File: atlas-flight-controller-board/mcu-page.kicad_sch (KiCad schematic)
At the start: 5 parts, among them J1 LED Indicator Header, J4 5V Input Power, U2 DEV-16771

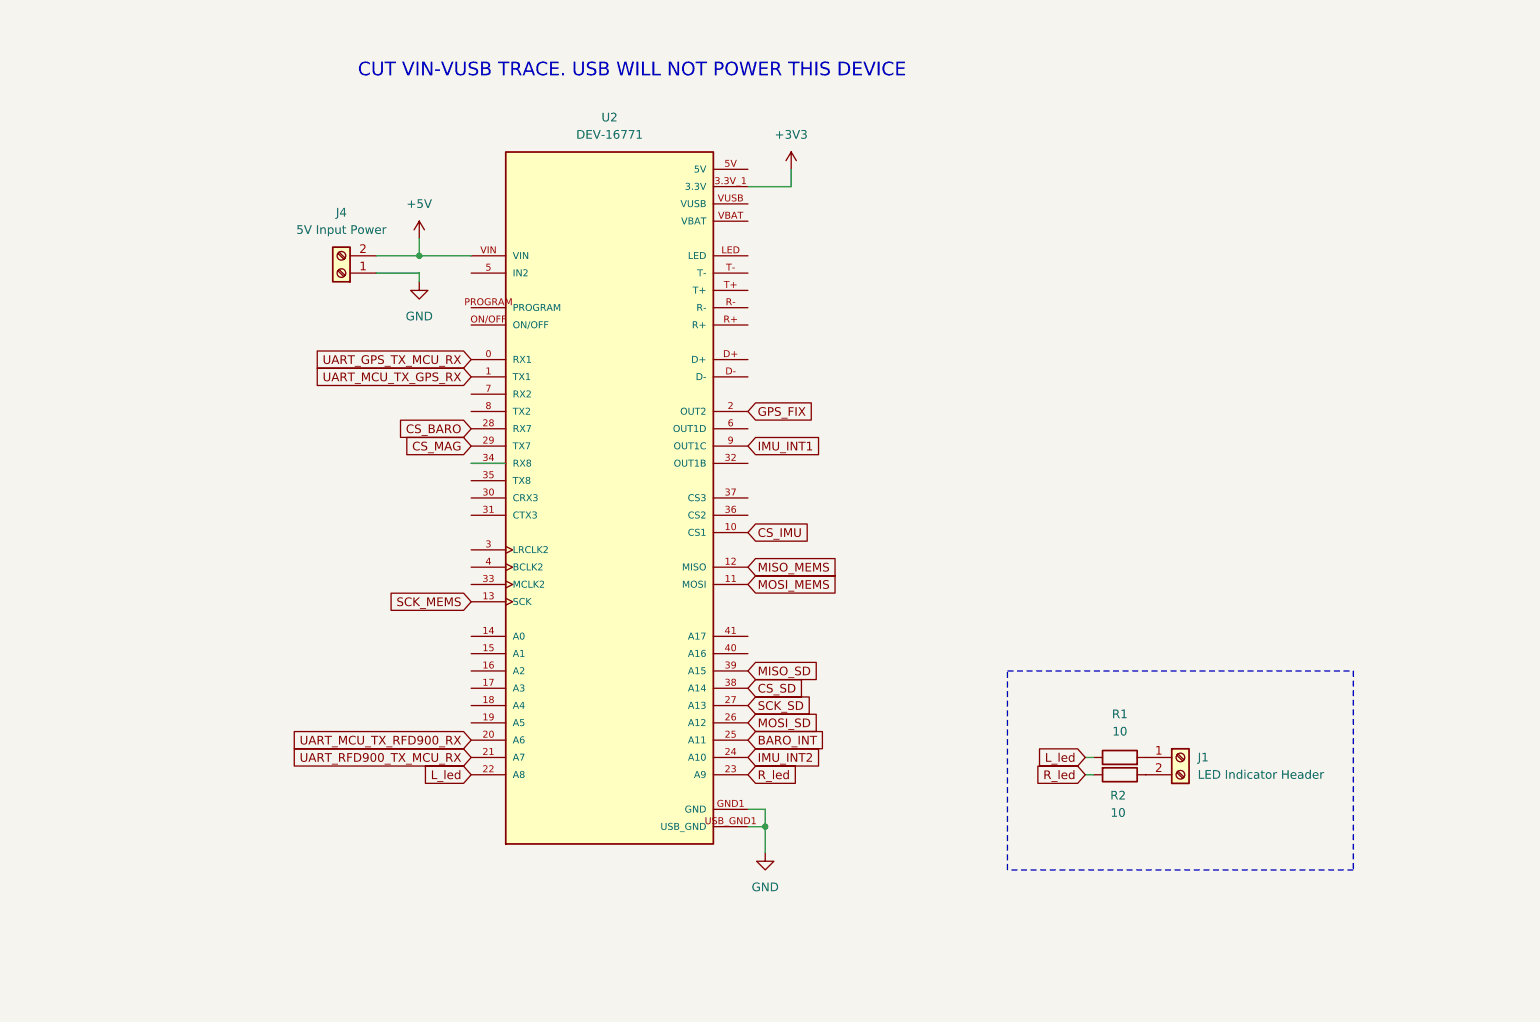
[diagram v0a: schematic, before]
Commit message: Done.
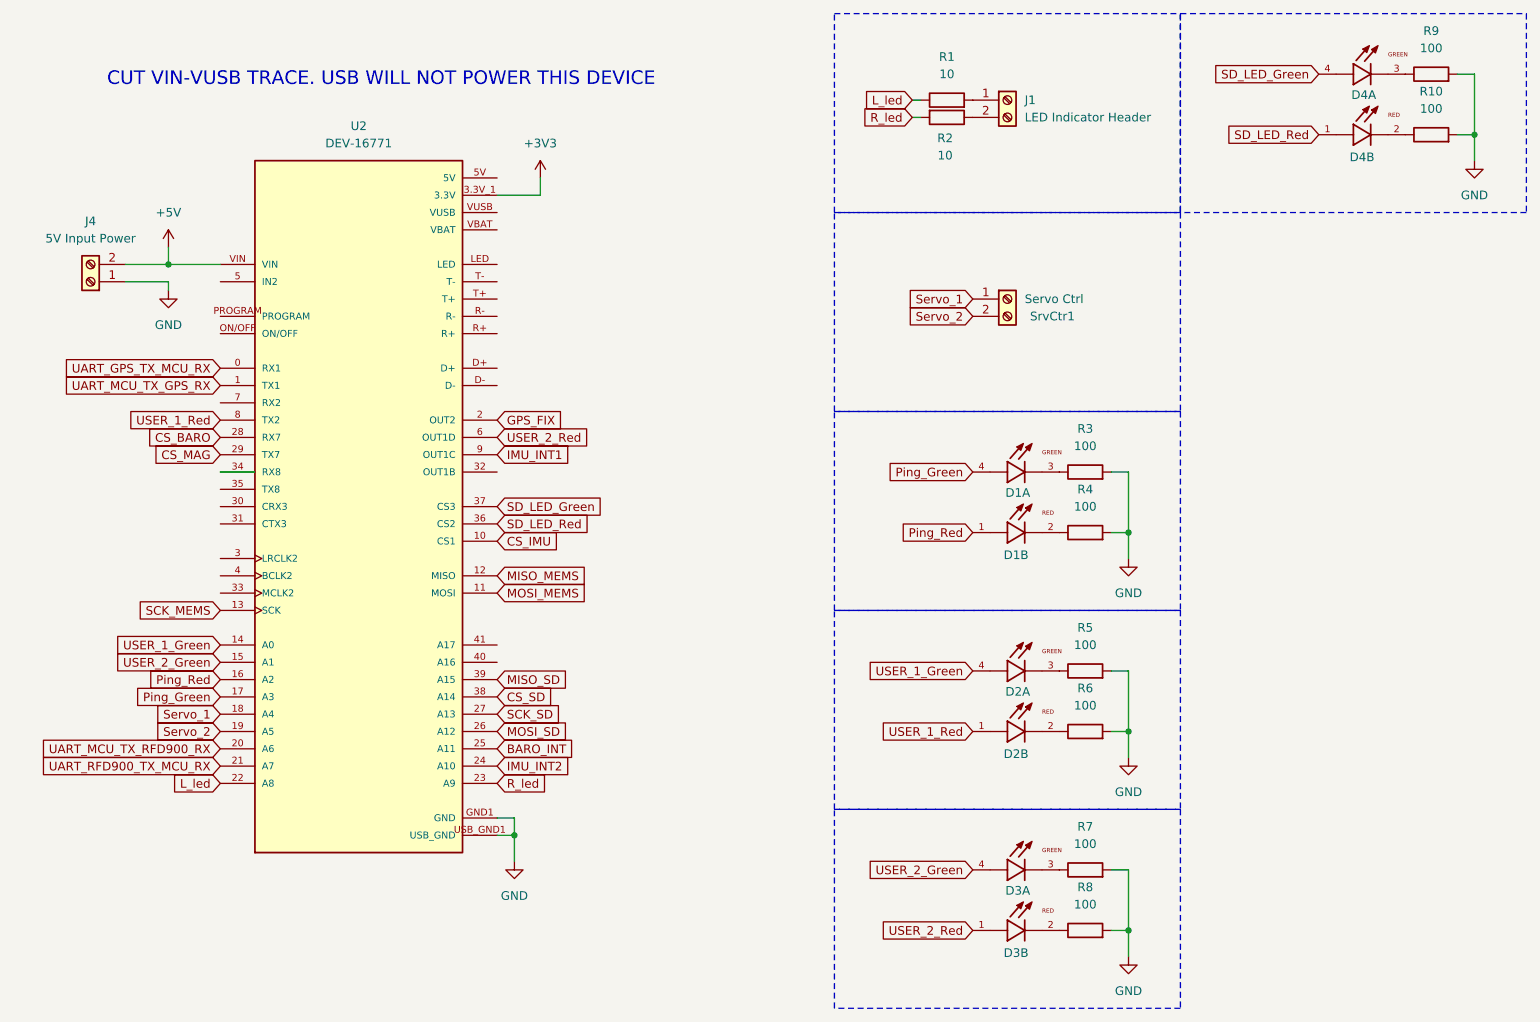
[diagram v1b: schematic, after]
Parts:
- added D1, D2, D3, D4: APHBM2012LSURKZGKC, APHBM2012LSURKZGKC:LED_APHBM2012LSURKZGKC, symbol APHBM2012LSURKZGKC:APHBM2012LSURKZGKC
- added R10, R3, R4, R5, R6, R7, R8, R9: 100, Resistor_SMD:R_0603_1608Metric_Pad0.98x0.95mm_HandSolder, symbol Device:R
- added SrvCtr1: Servo Ctrl, TerminalBlock:TerminalBlock_Xinya_XY308-2.54-2P_1x02_P2.54mm_Horizontal, symbol Connector:Screw_Terminal_01x02
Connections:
- net GND: now also R10.2, R3.2, R4.2, R5.2, R6.2, R7.2, R8.2, R9.2
- net USER_1_Green: now reaches U2.14 (A0)
- net USER_1_Green: now also D2.4
- net USER_2_Green: now reaches U2.15 (A1)
- net USER_2_Green: now also D3.4
- net Ping_Red: now reaches U2.16 (A2)
- net Ping_Red: now also D1.1
- net Ping_Green: now reaches U2.17 (A3)
- net Ping_Green: now also D1.4
- net Servo_1: now reaches U2.18 (A4)
- net Servo_1: now also SrvCtr1.1 (Pin_1)
- net Servo_2: now reaches U2.19 (A5)
- net Servo_2: now also SrvCtr1.2 (Pin_2)
- net SD_LED_Red: now reaches U2.36 (CS2)
- net SD_LED_Red: now also D4.1
- net SD_LED_Green: now reaches U2.37 (CS3)
- net SD_LED_Green: now also D4.4
- net USER_2_Red: now reaches U2.6 (OUT1D)
- net USER_2_Red: now also D3.1
- net USER_1_Red: now reaches U2.8 (TX2)
- net USER_1_Red: now also D2.1
- new net: D2.2, R6.1
- new net: D3.3, R7.1
- new net: D4.3, R9.1
- new net: D1.2, R4.1
- new net: D2.3, R5.1
- new net: D4.2, R10.1
- new net: D1.3, R3.1
- new net: D3.2, R8.1
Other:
- moved on the sheet: J1, J4, R1, R2, U2
